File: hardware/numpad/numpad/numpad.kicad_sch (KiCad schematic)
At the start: 18 parts, among them U1 STM32F446RET6, Y1 8MHz

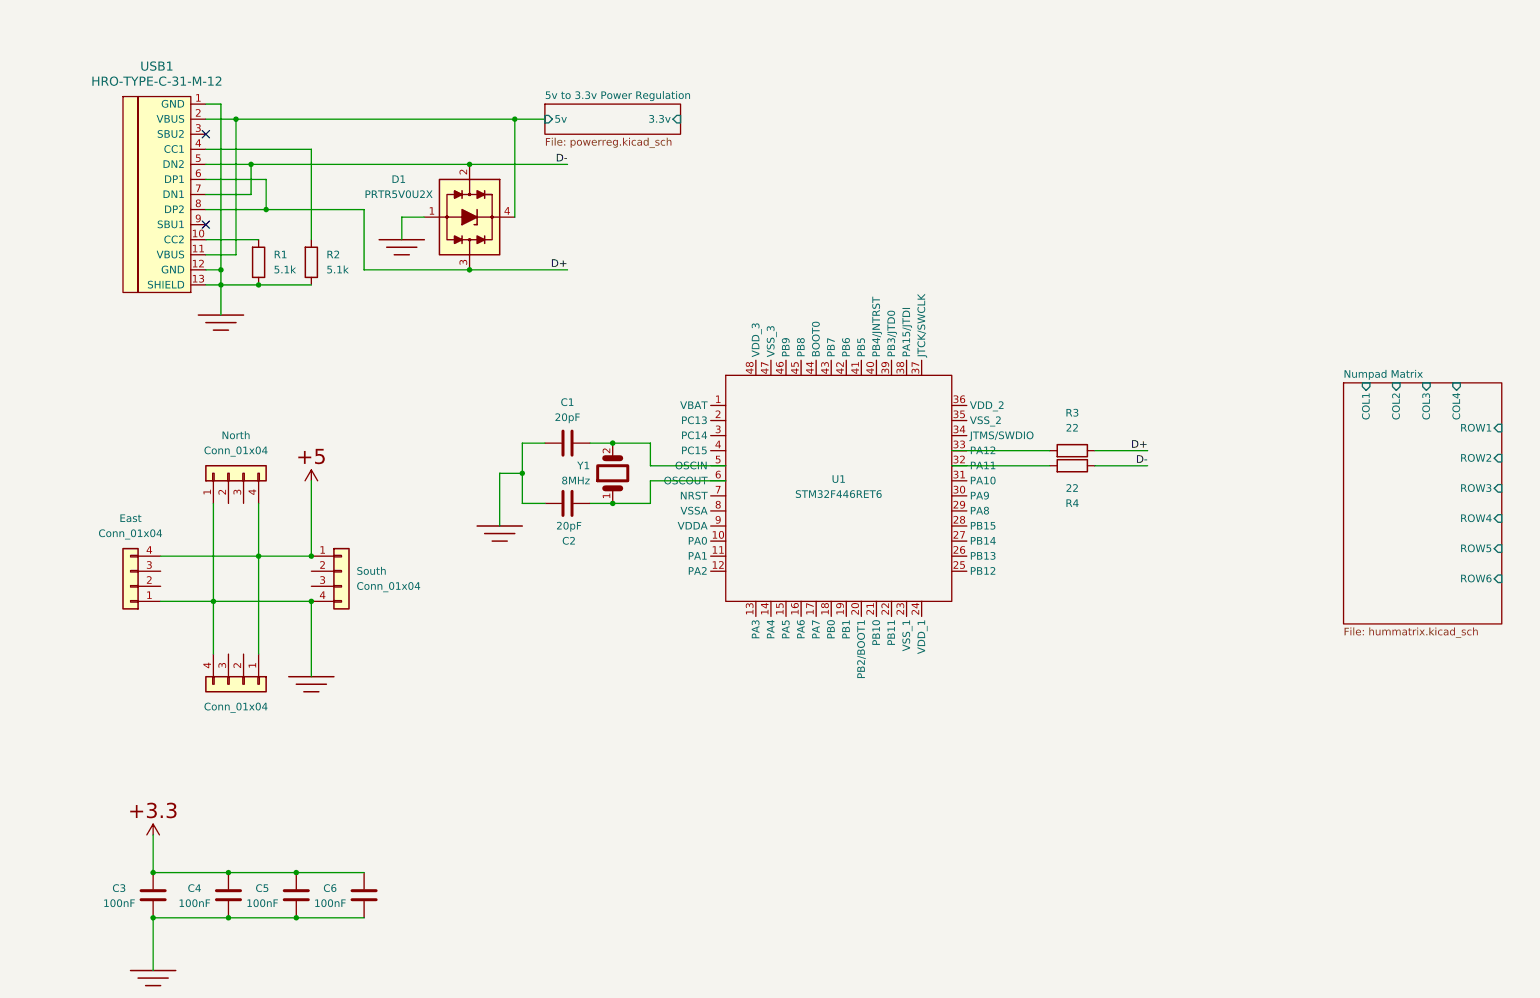
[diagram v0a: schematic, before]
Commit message: numpad, connections, and more
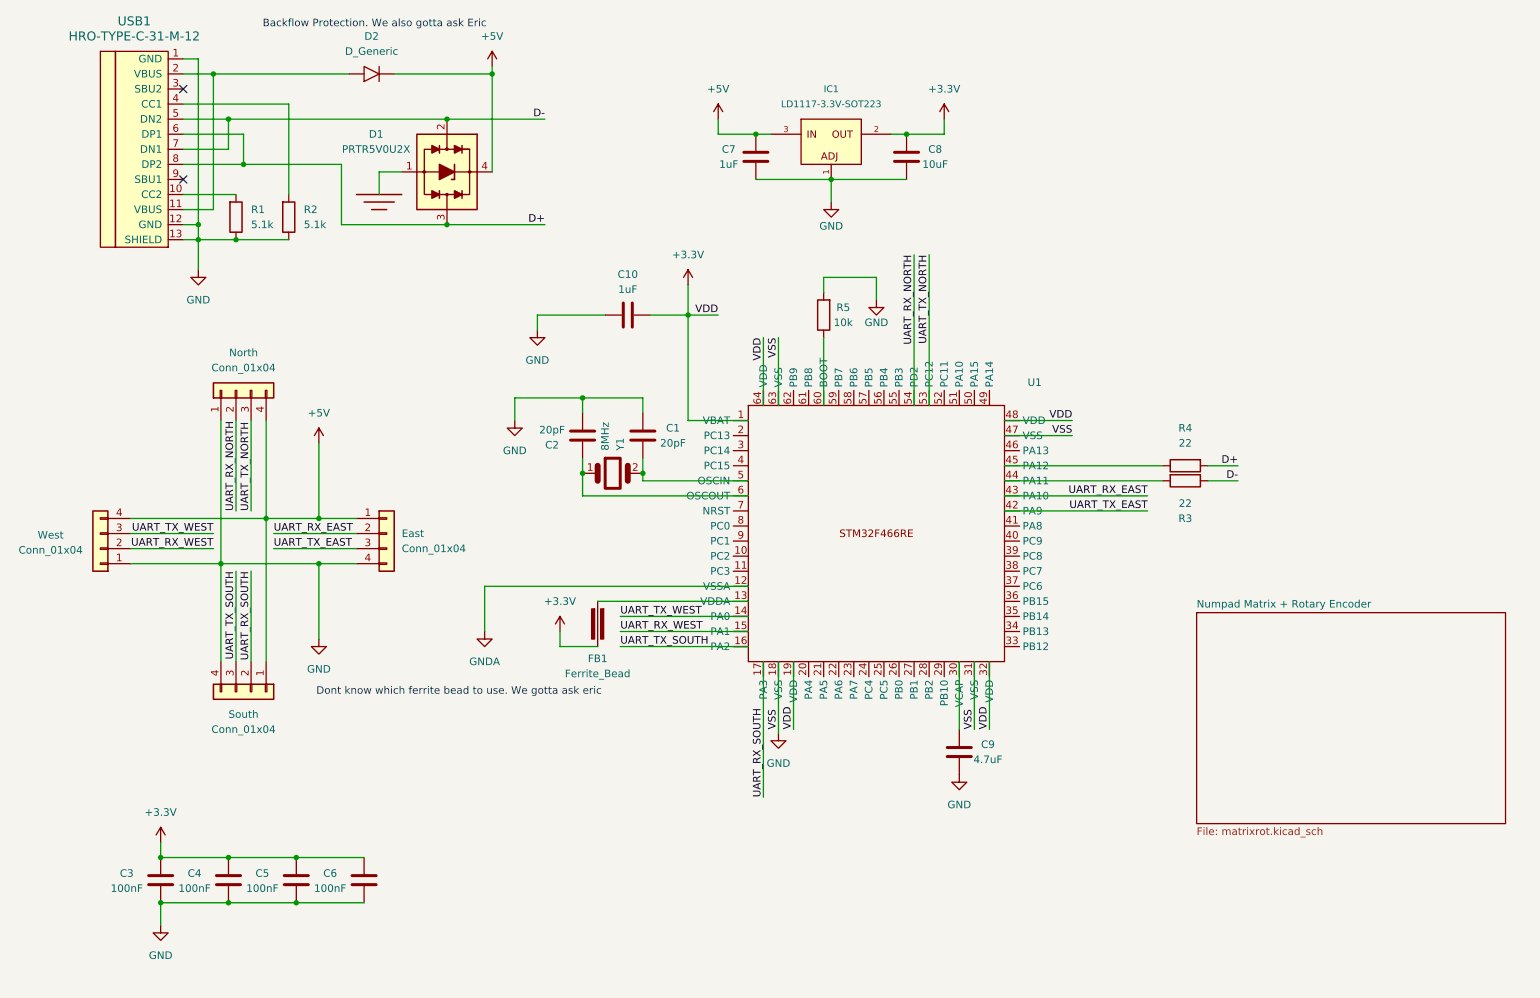
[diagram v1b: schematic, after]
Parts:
- removed West: Conn_01x04, 4ms_Connector:Pins_1x04_2.54mm_TH_SWD, symbol PCM_4ms_Connector:Conn_01x04
- added C10, C7: 1uF, PCM_Capacitor_SMD_AKL:C_0805_2012Metric, symbol PCM_Capacitor_AKL:C_0805
- added C8: 10uF, PCM_Capacitor_SMD_AKL:C_0805_2012Metric, symbol PCM_Capacitor_AKL:C_0805
- added C9: 4.7uF, PCM_Capacitor_SMD_AKL:C_0805_2012Metric, symbol PCM_Capacitor_AKL:C_0805
- added D2: D_Generic, symbol PCM_4ms_Diode:D_Generic
- added FB1: Ferrite_Bead, PCM_Fuse_AKL:Fuse_0805_2012Metric_Pad1.15x1.40mm_BigPads, symbol PCM_Device_AKL:Ferrite_Bead
- added IC1: LD1117-3.3V-SOT223, 4ms_Package_SOT:SOT223, symbol PCM_4ms_Regulator:LD1117-3.3V-SOT223
- added R5: 10k, PCM_Resistor_SMD_AKL:R_0805_2012Metric, symbol PCM_Resistor_AKL:R_0805
- added South: Conn_01x04, 4ms_Connector:Pins_1x04_2.54mm_TH_SWD, symbol PCM_4ms_Connector:Conn_01x04
- U1: value STM32F446RET6 -> ~; footprint footprints:LQFP64-10x10mm -> (none)
- renumbered South to East, East to West
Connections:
- net P,+3.3 is gone; now on net +3.3V: C3.1, C4.1, C5.1, C6.1
- net D+: now also R4.1; no longer R3.2
- net D-: now also R3.2; no longer R4.2
- net P,E: no longer C1.2, C2.2, C3.2, C4.2, C5.2, C6.2, East.4 (Pin_4), North.1 (Pin_1), R1.2, R2.2, USB1.1 (GND), USB1.12 (GND), USB1.13 (SHIELD), West.1 (Pin_1)
- net UART_RX_EAST: now reaches East.2 (Pin_2)
- net UART_RX_EAST: now also U1.43 (PA10)
- net UART_TX_EAST: now reaches East.3 (Pin_3)
- net UART_TX_EAST: now also U1.42 (PA9)
- net UART_RX_NORTH: now reaches North.2 (Pin_2)
- net UART_RX_NORTH: now also U1.54 (PD2)
- net UART_TX_NORTH: now reaches North.3 (Pin_3)
- net UART_TX_NORTH: now also U1.53 (PC12)
- net +3.3V: now reaches U1.32 (VDD)
- net +3.3V: now also U1.1 (VBAT), U1.19 (VDD), U1.48 (VDD), U1.64 (VDD), C10.1, C8.2, FB1.2, IC1.2 (OUT); no longer R4.1
- net at U1.33 (PB12): no longer R3.1
- net GNDA: now reaches U1.12 (VSSA)
- net at U1.13 (VDDA): now also FB1.1
- net UART_TX_WEST: now reaches U1.14 (PA0)
- net UART_TX_WEST: now also West.3 (Pin_3)
- net UART_RX_WEST: now reaches U1.15 (PA1)
- net UART_RX_WEST: now also West.2 (Pin_2)
- net UART_TX_SOUTH: now reaches U1.16 (PA2)
- net UART_TX_SOUTH: now also South.3 (Pin_3)
- net UART_RX_SOUTH: now reaches U1.17 (PA3)
- net UART_RX_SOUTH: now also South.2 (Pin_2)
- net GND: now reaches U1.18 (VSS)
- net GND: now also C1.2, C2.2, C3.2, C4.2, C5.2, C6.2, East.4 (Pin_4), North.1 (Pin_1), R1.2, R2.2, U1.31 (VSS), U1.47 (VSS), U1.63 (VSS), USB1.1 (GND), USB1.12 (GND), USB1.13 (SHIELD), West.1 (Pin_1), C10.2, C7.2, C8.1, C9.1, IC1.1 (ADJ), R5.1, South.4 (Pin_4)
- net at U1.30 (VCAP): now also C9.2
- net at U1.44 (PA11): now also R3.1
- net at U1.45 (PA12): now also R4.2
- net 5v to 3.3v Power Regulation/5v: no longer names the net of USB1.11 (VBUS), USB1.2 (VBUS)
- net 5v to 3.3v Power Regulation/5v: now also D2.2 (A); no longer D1.4 (VP)
- net P,+5 renamed +5V
- net +5V: now also D1.4 (VP), C7.1, D2.1 (K), IC1.3 (IN), South.1 (Pin_1)
- new net: R5.2, U1.60 (BOOT)
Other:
- removed sheet 5v to 3.3v Power Regulation
- removed sheet Numpad Matrix
- added sheet Numpad Matrix + Rotary Encoder (matrixrot.kicad_sch)
- note added: "Backflow Protection. We also gotta ask Eric"
- note added: "Dont know which ferrite bead to use. We gotta ask eric"
- moved on the sheet: C1, C2, C3, C4, C5, C6, D1, East, North, R1, R2, R3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
